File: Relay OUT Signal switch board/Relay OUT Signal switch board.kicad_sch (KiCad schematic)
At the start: 24 parts, among them IC1 ULN2003LVDR, J1 1725669, J10 1725669, J12 1725669, J13 1725669, J14 1725669, J15 1725669, J16 1725669, J17 1725669, J18 1725669, J19 1725669, J3 1725669, K1 EC2-5SNU, K2 EC2-5SNU, K3 EC2-5SNU

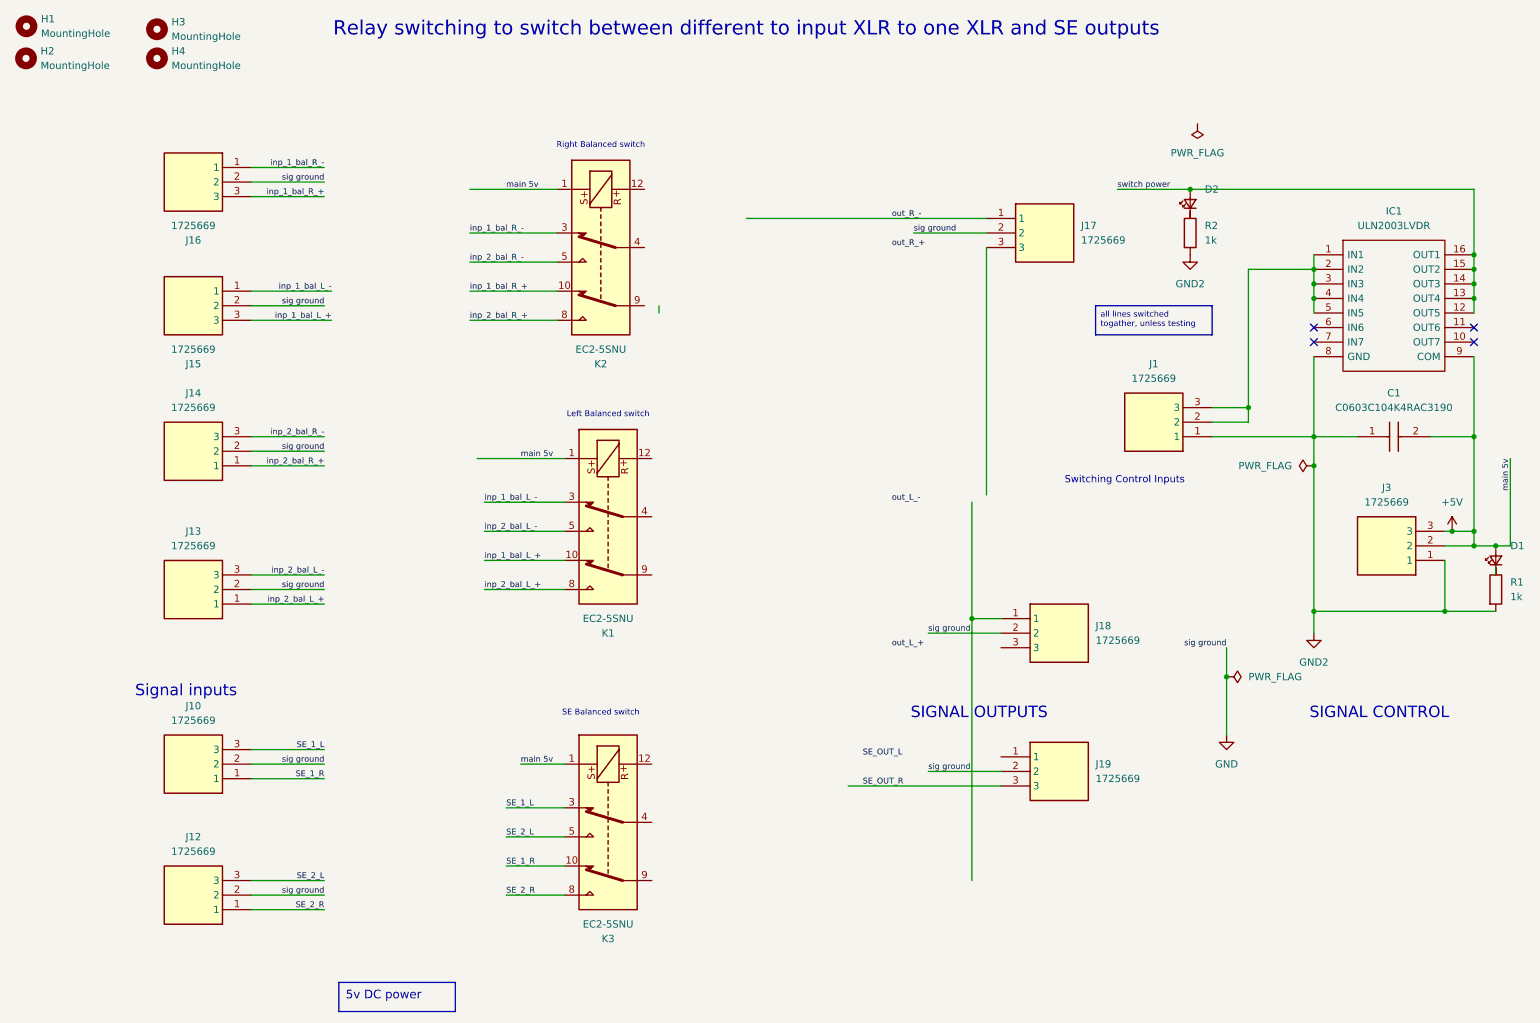
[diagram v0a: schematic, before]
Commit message: updated final four boards for streamer
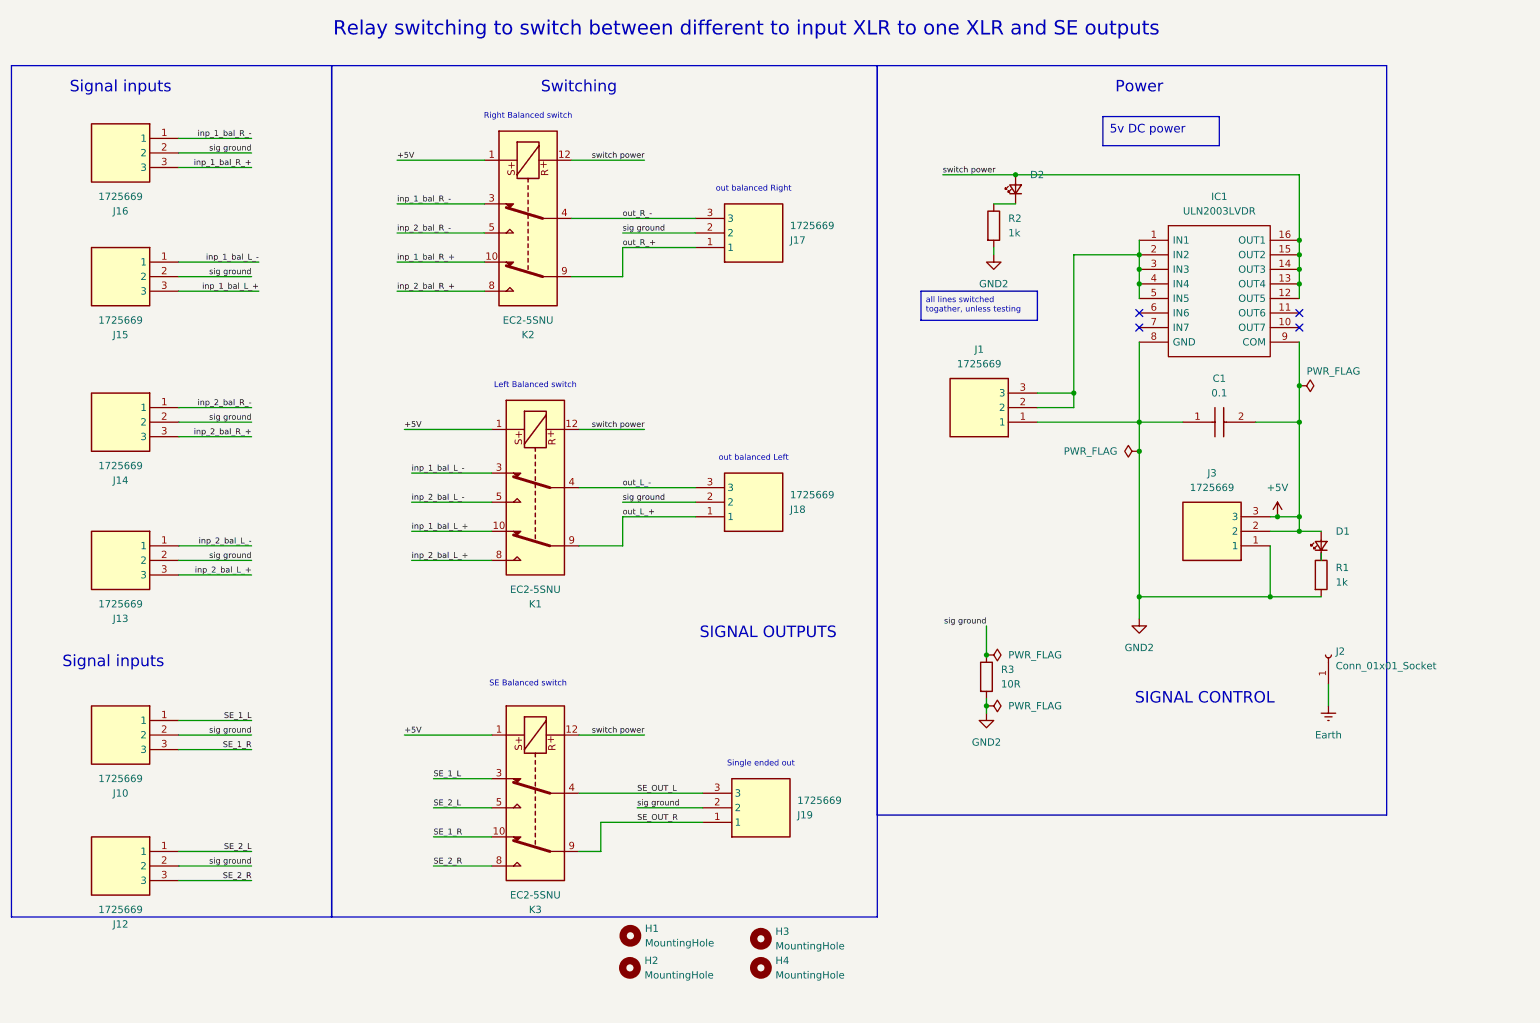
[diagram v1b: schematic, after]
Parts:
- added J2: Conn_01x01_Socket, Connector_PinHeader_1.00mm:PinHeader_1x01_P1.00mm_Vertical, symbol Connector:Conn_01x01_Socket
- added R3: 10R, Resistor_SMD:R_0603_1608Metric, symbol Device:R
- C1: value C0603C104K4RAC3190 -> 0.1
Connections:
- net GND2: now also R3.2
- net SE_1_L: now also J10.1; no longer J10.3
- net SE_1_R: now also J10.3; no longer J10.1
- net SE_2_L: now also J12.1; no longer J12.3
- net SE_2_R: now also J12.3; no longer J12.1
- net SE_OUT_L: now also J19.3, K3.4
- net SE_OUT_R: now also J19.1, K3.9; no longer J19.3
- net inp_2_bal_L_+: now also J13.3; no longer J13.1
- net inp_2_bal_L_-: now also J13.1; no longer J13.3
- net inp_2_bal_R_+: now also J14.3; no longer J14.1
- net inp_2_bal_R_-: now also J14.1; no longer J14.3
- net out_L_+: now also J18.1, K1.9
- net out_L_-: now also J18.3, K1.4
- net out_R_+: now also J17.1, K2.9
- net out_R_-: now also J17.3, K2.4; no longer J17.1
- net switch power: now also K1.12, K2.12, K3.12
- net at R2.1: now also D2.1 (K)
- net GND renamed sig ground
- net sig ground: now also R3.1
- new net Earth: J2.1 (Pin_1)
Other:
- note added: "Power"
- note added: "Single ended out"
- note added: "Switching"
- note added: "out balanced Left"
- note added: "out balanced Right"
- note removed: "Switching Control Inputs"
- moved on the sheet: C1, D1, D2, H1, H2, H3, H4, IC1, J1, J10, J12, J13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
